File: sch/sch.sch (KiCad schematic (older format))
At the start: 27 parts, among them J1 swd, J2 JOY_CON, J3 USB, J4 JOYSTICK, SW1 SW_LEFT, SW2 SW_UP, SW3 SW_RIGHT, SW4 SW_DOWN, SW5 SW_1, SW6 SW_2, U1 STM32F103C8Tx_usb, U2 XC6206-33, Y1 8M

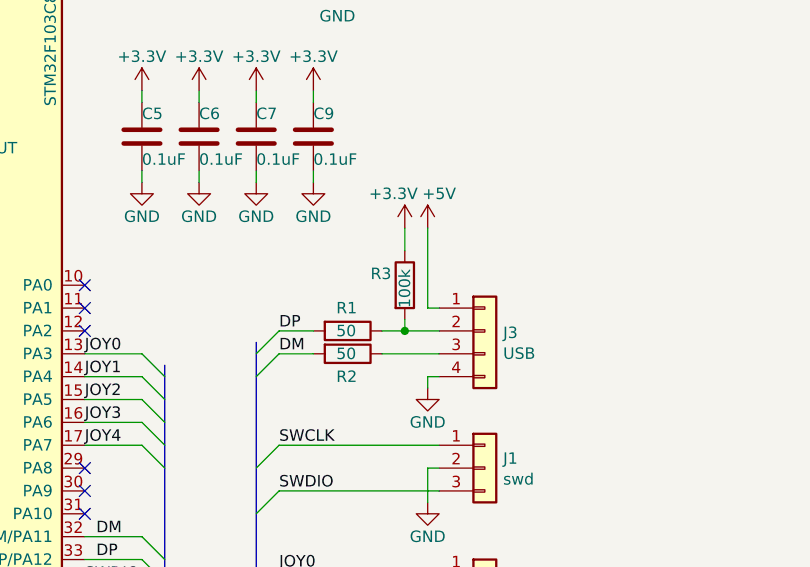
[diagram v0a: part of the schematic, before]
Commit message: begin to write normal documentation
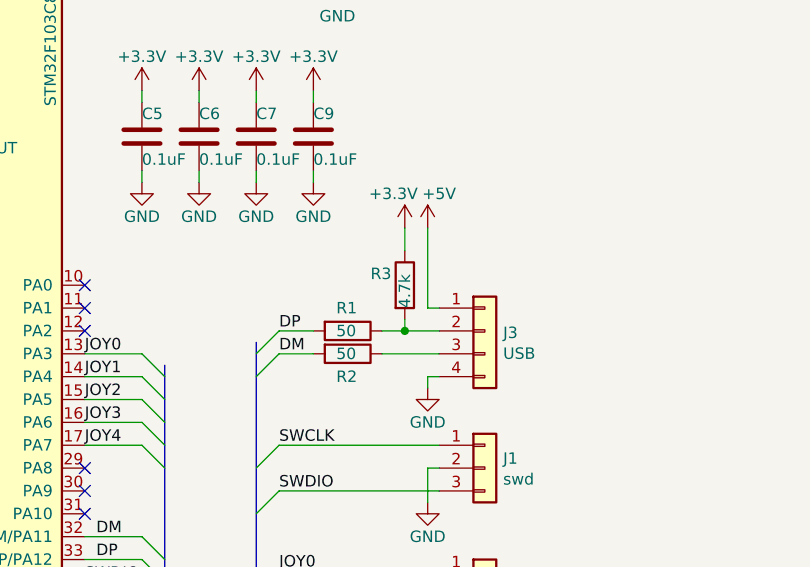
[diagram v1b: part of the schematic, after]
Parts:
- R3: value 100k -> 4.7k
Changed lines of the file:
@@
 P 6950 3500
 F 0 "R3" H 6800 3550 50  0000 L CNN
-F 1 "100k" V 6950 3400 50  0000 L CNN
+F 1 "4.7k" V 6950 3400 50  0000 L CNN
 F 2 "Resistor_SMD:R_0402_1005Metric" V 6880 3500 50  0001 C CNN
 F 3 "" H 6950 3500 50  0001 C CNN

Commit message: *
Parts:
- C1, C10, C2, C3, C4, C5, C6, C7, C8, C9: symbol device:C -> sch-rescue:C-device
- J1: symbol Connector:Conn_01x03 -> sch-rescue:Conn_01x03-Connector
- J2: symbol Connector:Conn_01x09 -> sch-rescue:Conn_01x09-Connector
- J3: symbol Connector:Conn_01x04 -> sch-rescue:Conn_01x04-Connector
- J4: symbol Connector:Conn_01x07 -> sch-rescue:Conn_01x07-Connector
- R1, R2, R3, R4: symbol device:R -> sch-rescue:R-device
- SW1, SW2, SW3, SW4, SW5, SW6: symbol Switch:SW_Push -> sch-rescue:SW_Push-Switch
- Y1: symbol device:Crystal -> sch-rescue:Crystal-device
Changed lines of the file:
@@
 $EndDescr
 $Comp
-L device:R R3
+L sch-rescue:R-device R3
 U 1 1 60B98022
 P 6950 3500
@@
 $EndComp
 $Comp
-L power:+5V #PWR0101
+L sch-rescue:+5V-power #PWR0101
 U 1 1 60BA6D79
 P 7050 3250
@@
 $EndComp
 $Comp
-L device:Crystal Y1
+L sch-rescue:Crystal-device Y1
 U 1 1 60BB7B29
 P 4200 2850
@@
 $EndComp
 $Comp
-L device:C C1
+L sch-rescue:C-device C1
 U 1 1 60BBCAE9
 P 3900 2700
@@
 $EndComp
 $Comp
-L device:C C2
+L sch-rescue:C-device C2
 U 1 1 60BBD52B
 P 3900 3000
@@
 Connection ~ 4200 3000
 $Comp
-L power:GND #PWR0103
+L sch-rescue:GND-power #PWR0103
 U 1 1 60BC5327
 P 3650 3050
@@
 Connection ~ 3650 3000
 $Comp
-L device:C C5
+L sch-rescue:C-device C5
 U 1 1 60BCC99C
 P 5800 2850
@@
 $EndComp
 $Comp
-L power:GND #PWR0104
+L sch-rescue:GND-power #PWR0104
 U 1 1 60BCEBAF
 P 5800 3050
@@
 $EndComp
 $Comp
-L power:+3.3V #PWR0105
+L sch-rescue:+3.3V-power #PWR0105
 U 1 1 60BCF857
 P 5800 2650
@@
 $EndComp
 $Comp
-L device:C C6
+L sch-rescue:C-device C6
 U 1 1 60BD3987
 P 6050 2850
@@
 $EndComp
 $Comp
-L power:GND #PWR0106
+L sch-rescue:GND-power #PWR0106
 U 1 1 60BD398D
 P 6050 3050
@@
 $EndComp
 $Comp
-L power:+3.3V #PWR0107
+L sch-rescue:+3.3V-power #PWR0107
 U 1 1 60BD3993
 P 6050 2650
@@
 $EndComp
 $Comp
-L device:C C7
+L sch-rescue:C-device C7
 U 1 1 60BD4708
 P 6300 2850
@@
 $EndComp
 $Comp
-L power:GND #PWR0108
+L sch-rescue:GND-power #PWR0108
 U 1 1 60BD470E
 P 6300 3050
@@
 $EndComp
 $Comp
-L power:+3.3V #PWR0109
+L sch-rescue:+3.3V-power #PWR0109
 U 1 1 60BD4714
 P 6300 2650
@@
 $EndComp
 $Comp
-L device:C C9
+L sch-rescue:C-device C9
 U 1 1 60BD5497
 P 6550 2850
@@
 $EndComp
 $Comp
-L power:GND #PWR0110
+L sch-rescue:GND-power #PWR0110
 U 1 1 60BD549D
 P 6550 3050
@@
 $EndComp
 $Comp
-L power:+3.3V #PWR0111
+L sch-rescue:+3.3V-power #PWR0111
 U 1 1 60BD54A3
 P 6550 2650
@@
 	6300 2650 6300 2700
 $Comp
-L power:+3.3V #PWR0112
+L sch-rescue:+3.3V-power #PWR0112
 U 1 1 60BE41C5
 P 5100 1700
@@
 Connection ~ 5100 1750
 $Comp
-L power:GND #PWR0113
+L sch-rescue:GND-power #PWR0113
 U 1 1 60BE8B74
 P 5100 5500
@@
 	4900 5450 5000 5450
 $Comp
-L power:GND #PWR0114
+L sch-rescue:GND-power #PWR0114
 U 1 1 60BFBFA2
 P 7050 3950
@@
 $EndComp
 $Comp
-L power:GND #PWR0115
+L sch-rescue:GND-power #PWR0115
 U 1 1 60C02E98
 P 4000 2400
@@
 $EndComp
 $Comp
-L device:C C3
+L sch-rescue:C-device C3
 U 1 1 60C06DEC
 P 4200 2200
@@
 $EndComp
 $Comp
-L power:GND #PWR0116
+L sch-rescue:GND-power #PWR0116
 U 1 1 60C0A725
 P 4000 2200
@@
 	4000 2400 4450 2400
 $Comp
-L power:+3.3V #PWR0117
+L sch-rescue:+3.3V-power #PWR0117
 U 1 1 60C17286
 P 4400 2550
@@
 	5900 5650 6000 5750
 $Comp
-L Connector:Conn_01x09 J2
+L sch-rescue:Conn_01x09-Connector J2
 U 1 1 60C72175
 P 7300 5150
@@
 JOY7
 $Comp
-L power:GND #PWR0118
+L sch-rescue:GND-power #PWR0118
 U 1 1 60CB8790
 P 7050 5600
@@
 	5700 1750 5700 1700
 $Comp
-L power:+3.3V #PWR0119
+L sch-rescue:+3.3V-power #PWR0119
 U 1 1 60BDEA7C
 P 5700 1700
@@
 $EndComp
 $Comp
-L power:+5V #PWR0120
+L sch-rescue:+5V-power #PWR0120
 U 1 1 60BDCB44
 P 7150 1700
@@
 	5700 2050 5700 2100
 $Comp
-L power:GND #PWR0121
+L sch-rescue:GND-power #PWR0121
 U 1 1 60BA3E87
 P 6650 2150
@@
 	5750 1750 5700 1750
 $Comp
-L device:C C8
+L sch-rescue:C-device C8
 U 1 1 60B9D265
 P 6400 1900
@@
 $EndComp
 $Comp
-L device:C C10
+L sch-rescue:C-device C10
 U 1 1 60B9CD1A
 P 6650 1900
@@
 $EndComp
 $Comp
-L device:C C4
+L sch-rescue:C-device C4
 U 1 1 60B9CA4E
 P 5700 1900
@@
 	6300 5650 6400 5750
 $Comp
-L device:R R2
+L sch-rescue:R-device R2
 U 1 1 60BAF8CE
 P 6700 3800
@@
 $EndComp
 $Comp
-L Connector:Conn_01x03 J1
+L sch-rescue:Conn_01x03-Connector J1
 U 1 1 60BDE5E6
 P 7300 4300
@@
 	6300 4500 6400 4400
 $Comp
-L power:GND #PWR0122
+L sch-rescue:GND-power #PWR0122
 U 1 1 60BEBAA9
 P 7050 4450
@@
 	5800 4800 5550 4800
 $Comp
-L device:R R4
+L sch-rescue:R-device R4
 U 1 1 60BAA748
 P 6950 1750
@@
 	7100 1750 7150 1750
 $Comp
-L Connector:Conn_01x04 J3
+L sch-rescue:Conn_01x04-Connector J3
 U 1 1 60BD2978
 P 7300 3700
@@
 	6300 3800 6400 3700
 $Comp
-L device:R R1
+L sch-rescue:R-device R1
 U 1 1 60BAF3EA
 P 6700 3700
@@
 NoConn ~ 4450 3300
 $Comp
-L power:GND #PWR0123
+L sch-rescue:GND-power #PWR0123
 U 1 1 60D66AD7
 P 4300 5050
@@
 NoConn ~ 5550 5000
 $Comp
-L Connector:Conn_01x07 J4
+L sch-rescue:Conn_01x07-Connector J4
 U 1 1 60E21F7B
 P 8200 5250
@@
 $EndComp
 $Comp
-L Switch:SW_Push SW6
+L sch-rescue:SW_Push-Switch SW6
 U 1 1 60E2AE97
 P 9000 5700
@@
 $EndComp
 $Comp
-L Switch:SW_Push SW5
+L sch-rescue:SW_Push-Switch SW5
 U 1 1 60E2BB79
 P 9000 5550
@@
 $EndComp
 $Comp
-L Switch:SW_Push SW4
+L sch-rescue:SW_Push-Switch SW4
 U 1 1 60E2DB4C
 P 9000 5400
@@
 $EndComp
 $Comp
-L Switch:SW_Push SW3
+L sch-rescue:SW_Push-Switch SW3
 U 1 1 60E2DDFE
 P 9000 5250
@@
 $EndComp
 $Comp
-L Switch:SW_Push SW2
+L sch-rescue:SW_Push-Switch SW2
 U 1 1 60E2E03E
 P 9000 5100
@@
 $EndComp
 $Comp
-L Switch:SW_Push SW1
+L sch-rescue:SW_Push-Switch SW1
 U 1 1 60E2E395
 P 9000 4950
@@
 	7050 3250 7050 3600
 $Comp
-L power:+3.3V #PWR0102
+L sch-rescue:+3.3V-power #PWR0102
 U 1 1 6105D4FC
 P 6950 3250

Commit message: убрался в файлах
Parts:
- C1, C10, C2, C3, C4, C5, C6, C7, C8, C9: symbol sch-rescue:C-device -> sch-rescue:C-device-sch-rescue
- J1: symbol sch-rescue:Conn_01x03-Connector -> sch-rescue:Conn_01x03-Connector-sch-rescue
- J2: symbol sch-rescue:Conn_01x09-Connector -> sch-rescue:Conn_01x09-Connector-sch-rescue
- J3: symbol sch-rescue:Conn_01x04-Connector -> sch-rescue:Conn_01x04-Connector-sch-rescue
- J4: symbol sch-rescue:Conn_01x07-Connector -> sch-rescue:Conn_01x07-Connector-sch-rescue
- R1, R2, R3, R4: symbol sch-rescue:R-device -> sch-rescue:R-device-sch-rescue
- SW1, SW2, SW3, SW4, SW5, SW6: symbol sch-rescue:SW_Push-Switch -> sch-rescue:SW_Push-Switch-sch-rescue
- Y1: symbol sch-rescue:Crystal-device -> sch-rescue:Crystal-device-sch-rescue
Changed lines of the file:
@@
 $EndDescr
 $Comp
-L sch-rescue:R-device R3
+L sch-rescue:R-device-sch-rescue R3
 U 1 1 60B98022
 P 6950 3500
@@
 $EndComp
 $Comp
-L sch-rescue:+5V-power #PWR0101
+L sch-rescue:+5V-power-sch-rescue #PWR0101
 U 1 1 60BA6D79
 P 7050 3250
@@
 $EndComp
 $Comp
-L sch-rescue:Crystal-device Y1
+L sch-rescue:Crystal-device-sch-rescue Y1
 U 1 1 60BB7B29
 P 4200 2850
@@
 $EndComp
 $Comp
-L sch-rescue:C-device C1
+L sch-rescue:C-device-sch-rescue C1
 U 1 1 60BBCAE9
 P 3900 2700
@@
 $EndComp
 $Comp
-L sch-rescue:C-device C2
+L sch-rescue:C-device-sch-rescue C2
 U 1 1 60BBD52B
 P 3900 3000
@@
 Connection ~ 4200 3000
 $Comp
-L sch-rescue:GND-power #PWR0103
+L sch-rescue:GND-power-sch-rescue #PWR0103
 U 1 1 60BC5327
 P 3650 3050
@@
 Connection ~ 3650 3000
 $Comp
-L sch-rescue:C-device C5
+L sch-rescue:C-device-sch-rescue C5
 U 1 1 60BCC99C
 P 5800 2850
@@
 $EndComp
 $Comp
-L sch-rescue:GND-power #PWR0104
+L sch-rescue:GND-power-sch-rescue #PWR0104
 U 1 1 60BCEBAF
 P 5800 3050
@@
 $EndComp
 $Comp
-L sch-rescue:+3.3V-power #PWR0105
+L sch-rescue:+3.3V-power-sch-rescue #PWR0105
 U 1 1 60BCF857
 P 5800 2650
@@
 $EndComp
 $Comp
-L sch-rescue:C-device C6
+L sch-rescue:C-device-sch-rescue C6
 U 1 1 60BD3987
 P 6050 2850
@@
 $EndComp
 $Comp
-L sch-rescue:GND-power #PWR0106
+L sch-rescue:GND-power-sch-rescue #PWR0106
 U 1 1 60BD398D
 P 6050 3050
@@
 $EndComp
 $Comp
-L sch-rescue:+3.3V-power #PWR0107
+L sch-rescue:+3.3V-power-sch-rescue #PWR0107
 U 1 1 60BD3993
 P 6050 2650
@@
 $EndComp
 $Comp
-L sch-rescue:C-device C7
+L sch-rescue:C-device-sch-rescue C7
 U 1 1 60BD4708
 P 6300 2850
@@
 $EndComp
 $Comp
-L sch-rescue:GND-power #PWR0108
+L sch-rescue:GND-power-sch-rescue #PWR0108
 U 1 1 60BD470E
 P 6300 3050
@@
 $EndComp
 $Comp
-L sch-rescue:+3.3V-power #PWR0109
+L sch-rescue:+3.3V-power-sch-rescue #PWR0109
 U 1 1 60BD4714
 P 6300 2650
@@
 $EndComp
 $Comp
-L sch-rescue:C-device C9
+L sch-rescue:C-device-sch-rescue C9
 U 1 1 60BD5497
 P 6550 2850
@@
 $EndComp
 $Comp
-L sch-rescue:GND-power #PWR0110
+L sch-rescue:GND-power-sch-rescue #PWR0110
 U 1 1 60BD549D
 P 6550 3050
@@
 $EndComp
 $Comp
-L sch-rescue:+3.3V-power #PWR0111
+L sch-rescue:+3.3V-power-sch-rescue #PWR0111
 U 1 1 60BD54A3
 P 6550 2650
@@
 	6300 2650 6300 2700
 $Comp
-L sch-rescue:+3.3V-power #PWR0112
+L sch-rescue:+3.3V-power-sch-rescue #PWR0112
 U 1 1 60BE41C5
 P 5100 1700
@@
 Connection ~ 5100 1750
 $Comp
-L sch-rescue:GND-power #PWR0113
+L sch-rescue:GND-power-sch-rescue #PWR0113
 U 1 1 60BE8B74
 P 5100 5500
@@
 	4900 5450 5000 5450
 $Comp
-L sch-rescue:GND-power #PWR0114
+L sch-rescue:GND-power-sch-rescue #PWR0114
 U 1 1 60BFBFA2
 P 7050 3950
@@
 $EndComp
 $Comp
-L sch-rescue:GND-power #PWR0115
+L sch-rescue:GND-power-sch-rescue #PWR0115
 U 1 1 60C02E98
 P 4000 2400
@@
 $EndComp
 $Comp
-L sch-rescue:C-device C3
+L sch-rescue:C-device-sch-rescue C3
 U 1 1 60C06DEC
 P 4200 2200
@@
 $EndComp
 $Comp
-L sch-rescue:GND-power #PWR0116
+L sch-rescue:GND-power-sch-rescue #PWR0116
 U 1 1 60C0A725
 P 4000 2200
@@
 	4000 2400 4450 2400
 $Comp
-L sch-rescue:+3.3V-power #PWR0117
+L sch-rescue:+3.3V-power-sch-rescue #PWR0117
 U 1 1 60C17286
 P 4400 2550
@@
 	5900 5650 6000 5750
 $Comp
-L sch-rescue:Conn_01x09-Connector J2
+L sch-rescue:Conn_01x09-Connector-sch-rescue J2
 U 1 1 60C72175
 P 7300 5150
@@
 JOY7
 $Comp
-L sch-rescue:GND-power #PWR0118
+L sch-rescue:GND-power-sch-rescue #PWR0118
 U 1 1 60CB8790
 P 7050 5600
@@
 	5700 1750 5700 1700
 $Comp
-L sch-rescue:+3.3V-power #PWR0119
+L sch-rescue:+3.3V-power-sch-rescue #PWR0119
 U 1 1 60BDEA7C
 P 5700 1700
@@
 $EndComp
 $Comp
-L sch-rescue:+5V-power #PWR0120
+L sch-rescue:+5V-power-sch-rescue #PWR0120
 U 1 1 60BDCB44
 P 7150 1700
@@
 	5700 2050 5700 2100
 $Comp
-L sch-rescue:GND-power #PWR0121
+L sch-rescue:GND-power-sch-rescue #PWR0121
 U 1 1 60BA3E87
 P 6650 2150
@@
 	5750 1750 5700 1750
 $Comp
-L sch-rescue:C-device C8
+L sch-rescue:C-device-sch-rescue C8
 U 1 1 60B9D265
 P 6400 1900
@@
 $EndComp
 $Comp
-L sch-rescue:C-device C10
+L sch-rescue:C-device-sch-rescue C10
 U 1 1 60B9CD1A
 P 6650 1900
@@
 $EndComp
 $Comp
-L sch-rescue:C-device C4
+L sch-rescue:C-device-sch-rescue C4
 U 1 1 60B9CA4E
 P 5700 1900
@@
 	6300 5650 6400 5750
 $Comp
-L sch-rescue:R-device R2
+L sch-rescue:R-device-sch-rescue R2
 U 1 1 60BAF8CE
 P 6700 3800
@@
 $EndComp
 $Comp
-L sch-rescue:Conn_01x03-Connector J1
+L sch-rescue:Conn_01x03-Connector-sch-rescue J1
 U 1 1 60BDE5E6
 P 7300 4300
@@
 	6300 4500 6400 4400
 $Comp
-L sch-rescue:GND-power #PWR0122
+L sch-rescue:GND-power-sch-rescue #PWR0122
 U 1 1 60BEBAA9
 P 7050 4450
@@
 	5800 4800 5550 4800
 $Comp
-L sch-rescue:R-device R4
+L sch-rescue:R-device-sch-rescue R4
 U 1 1 60BAA748
 P 6950 1750
@@
 	7100 1750 7150 1750
 $Comp
-L sch-rescue:Conn_01x04-Connector J3
+L sch-rescue:Conn_01x04-Connector-sch-rescue J3
 U 1 1 60BD2978
 P 7300 3700
@@
 	6300 3800 6400 3700
 $Comp
-L sch-rescue:R-device R1
+L sch-rescue:R-device-sch-rescue R1
 U 1 1 60BAF3EA
 P 6700 3700
@@
 NoConn ~ 4450 3300
 $Comp
-L sch-rescue:GND-power #PWR0123
+L sch-rescue:GND-power-sch-rescue #PWR0123
 U 1 1 60D66AD7
 P 4300 5050
@@
 NoConn ~ 5550 5000
 $Comp
-L sch-rescue:Conn_01x07-Connector J4
+L sch-rescue:Conn_01x07-Connector-sch-rescue J4
 U 1 1 60E21F7B
 P 8200 5250
@@
 $EndComp
 $Comp
-L sch-rescue:SW_Push-Switch SW6
+L sch-rescue:SW_Push-Switch-sch-rescue SW6
 U 1 1 60E2AE97
 P 9000 5700
@@
 $EndComp
 $Comp
-L sch-rescue:SW_Push-Switch SW5
+L sch-rescue:SW_Push-Switch-sch-rescue SW5
 U 1 1 60E2BB79
 P 9000 5550
@@
 $EndComp
 $Comp
-L sch-rescue:SW_Push-Switch SW4
+L sch-rescue:SW_Push-Switch-sch-rescue SW4
 U 1 1 60E2DB4C
 P 9000 5400
@@
 $EndComp
 $Comp
-L sch-rescue:SW_Push-Switch SW3
+L sch-rescue:SW_Push-Switch-sch-rescue SW3
 U 1 1 60E2DDFE
 P 9000 5250
@@
 $EndComp
 $Comp
-L sch-rescue:SW_Push-Switch SW2
+L sch-rescue:SW_Push-Switch-sch-rescue SW2
 U 1 1 60E2E03E
 P 9000 5100
@@
 $EndComp
 $Comp
-L sch-rescue:SW_Push-Switch SW1
+L sch-rescue:SW_Push-Switch-sch-rescue SW1
 U 1 1 60E2E395
 P 9000 4950
@@
 	7050 3250 7050 3600
 $Comp
-L sch-rescue:+3.3V-power #PWR0102
+L sch-rescue:+3.3V-power-sch-rescue #PWR0102
 U 1 1 6105D4FC
 P 6950 3250
